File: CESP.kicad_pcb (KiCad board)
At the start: 2 copper layers, 55.9 x 44.7 mm, 9 parts

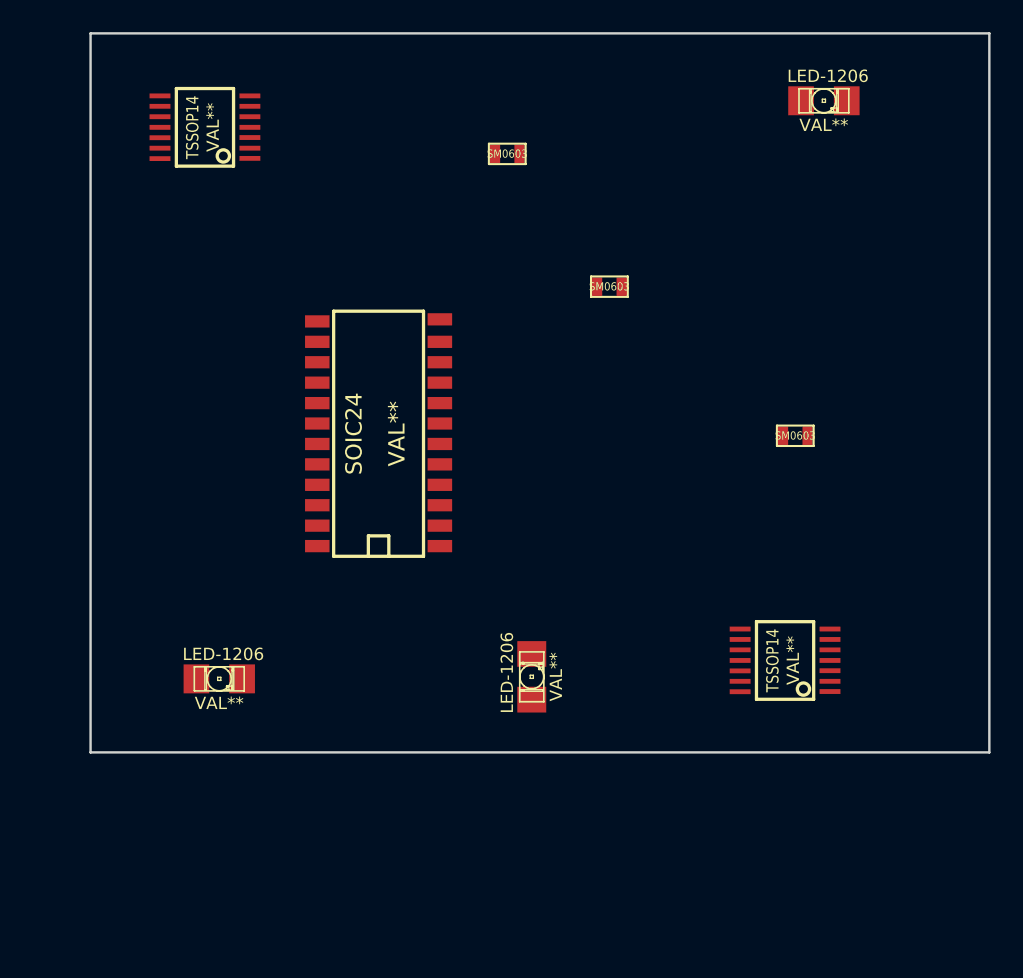
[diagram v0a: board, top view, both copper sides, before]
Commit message: second commit
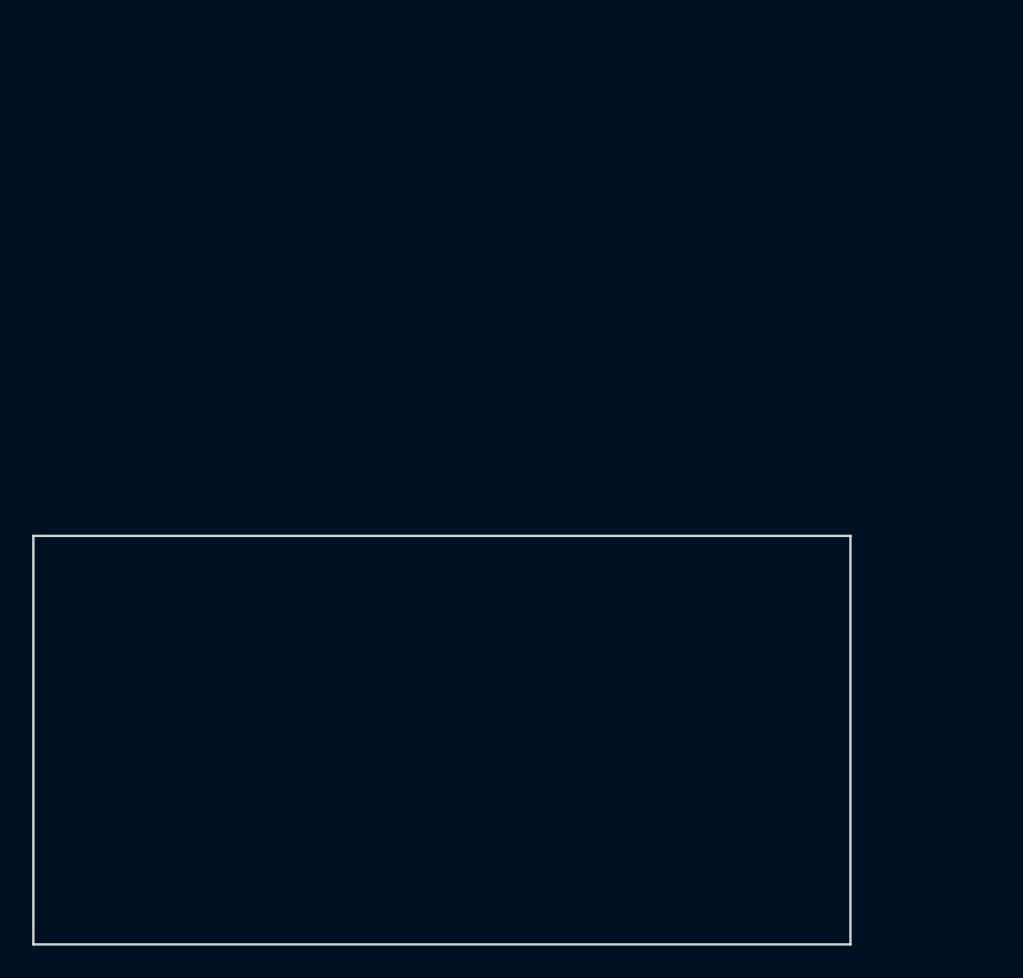
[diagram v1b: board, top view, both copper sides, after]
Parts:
- removed LED-1206 (x3): VAL**, LED-1206
- removed SM0603 (x3): Val**, SM0603
- removed SOIC24: VAL**, SOIC24
- removed TSSOP14 (x2): VAL**, TSSOP14
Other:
- board size 55.9 x 44.7 mm -> 50.8 x 25.4 mm
- board text removed: "NOTE: THIS IS JUST A TEST BOARD REMOVE ALL COMPONENTS AND CREATE YOUR OWN INCLUDE SCHEMATIC HOOKUPS/NETLIST"
